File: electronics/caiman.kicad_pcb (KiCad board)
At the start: 2 copper layers, 90.9 x 93.9 mm, 134 parts, among them J1 Conn_01x03_Pin, J10 Conn_01x04_Pin, J11 Conn_01x04_Pin, J12 Conn_01x04_Pin, J13 Micro_SD_Card, J14 50 ohm, J15 Conn_01x03_Pin, J2 Conn_01x04_Pin, J3 Conn_01x04_Pin, J4 Conn_01x03_Pin, J5 Conn_01x04_Pin, J6 Conn_01x04_Pin, J7 Conn_01x02_Pin, J8 Conn_01x02_Pin, J9 Conn_01x02_Pin, Q1 Q_PMOS-E_Generic_SSSGD, Q2 AON6262E, U1 AP63205WU, U10 SN74LV1T34DBV, U2 AP63203WU, U3 US1881, U4 LM74700, U5 LPS22HBTR, U6 LIS2MDLTR, U7 STM32F765VITx, U8 LSM6DSO, U9 nRF24L01P, Y1 8MHz, Y2 16MHz

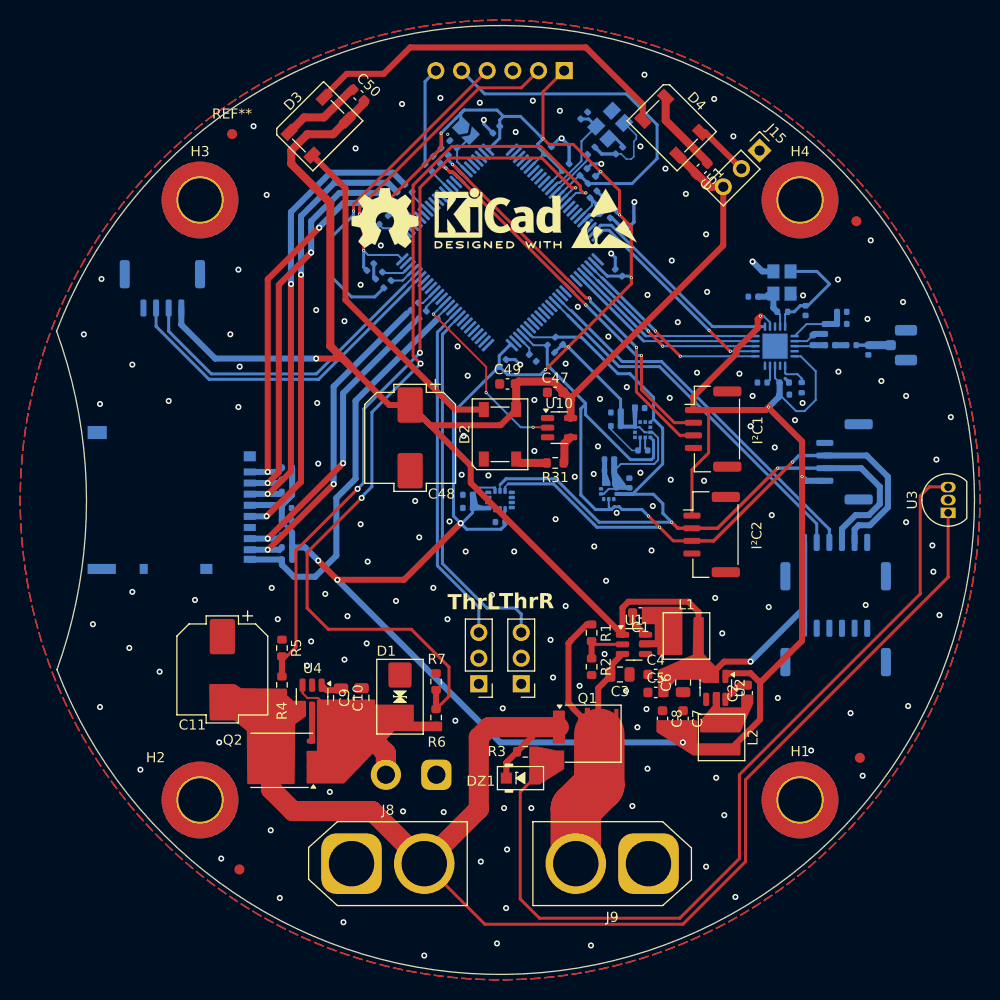
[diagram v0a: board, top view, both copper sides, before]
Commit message: Finalization of PCB
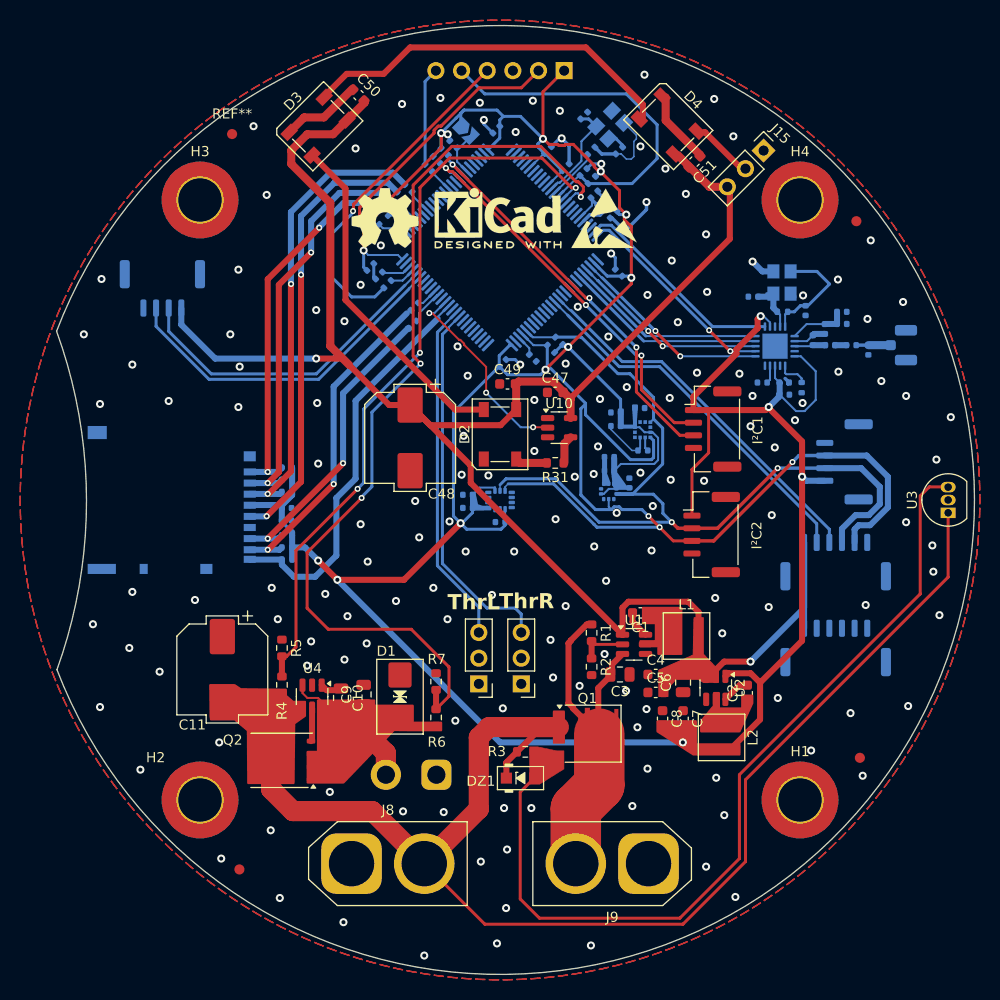
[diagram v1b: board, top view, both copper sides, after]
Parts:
- moved R22 1.38 mm to (141.4, 82.6)
- moved C51 1.02 mm to (169.2, 66.5)
- moved J15 0.40 mm to (176.1, 65.4)
- moved C9 0.39 mm to (136.5, 119.2)
- moved D4 0.37 mm to (166.6, 62.9)
- moved C22 0.25 mm to (160.8, 95.8)
- moved C21 0.09 mm to (159.3, 69.8)
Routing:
- net Net-(U7-PC8): track 2.06 -> 3.50 mm
- net +3V3: track 328.6 -> 329.6 mm
- net /LED: track 19.1 -> 20.0 mm
- net /DAT0: track 30.9 -> 30.0 mm
- net +5V: track 190.4 -> 191.0 mm
- net GND: track 45.9 -> 45.4 mm
